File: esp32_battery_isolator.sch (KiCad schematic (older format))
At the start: 78 parts, among them J1 BATT1, J2 Conn_01x04_Female, J3 USB_B_Micro, J4 BATT2, J5 LOAD1, J6 CHGR, J7 LOAD2, J8 LOAD3, J9 Conn_01x03_Male, Q1 MMBT3904, Q10 AONR21321, Q11 AONR21321, Q12 MMBT3904, Q13 AONR21321, Q2 AONR21321, Q3 MMBT3904, Q4 AONR21321, Q5 MMBT3904, Q6 AONR21321, Q7 MMBT3904, Q8 AONR21321, Q9 MMBT3904, SW1 C492887, SW2 C492887, U1 ESP32-WROOM-32D, U3 ADC128D818, U4 CC6903SO-30A, U5 CH330N, U6 CC6903SO-30A, U7 BL9342

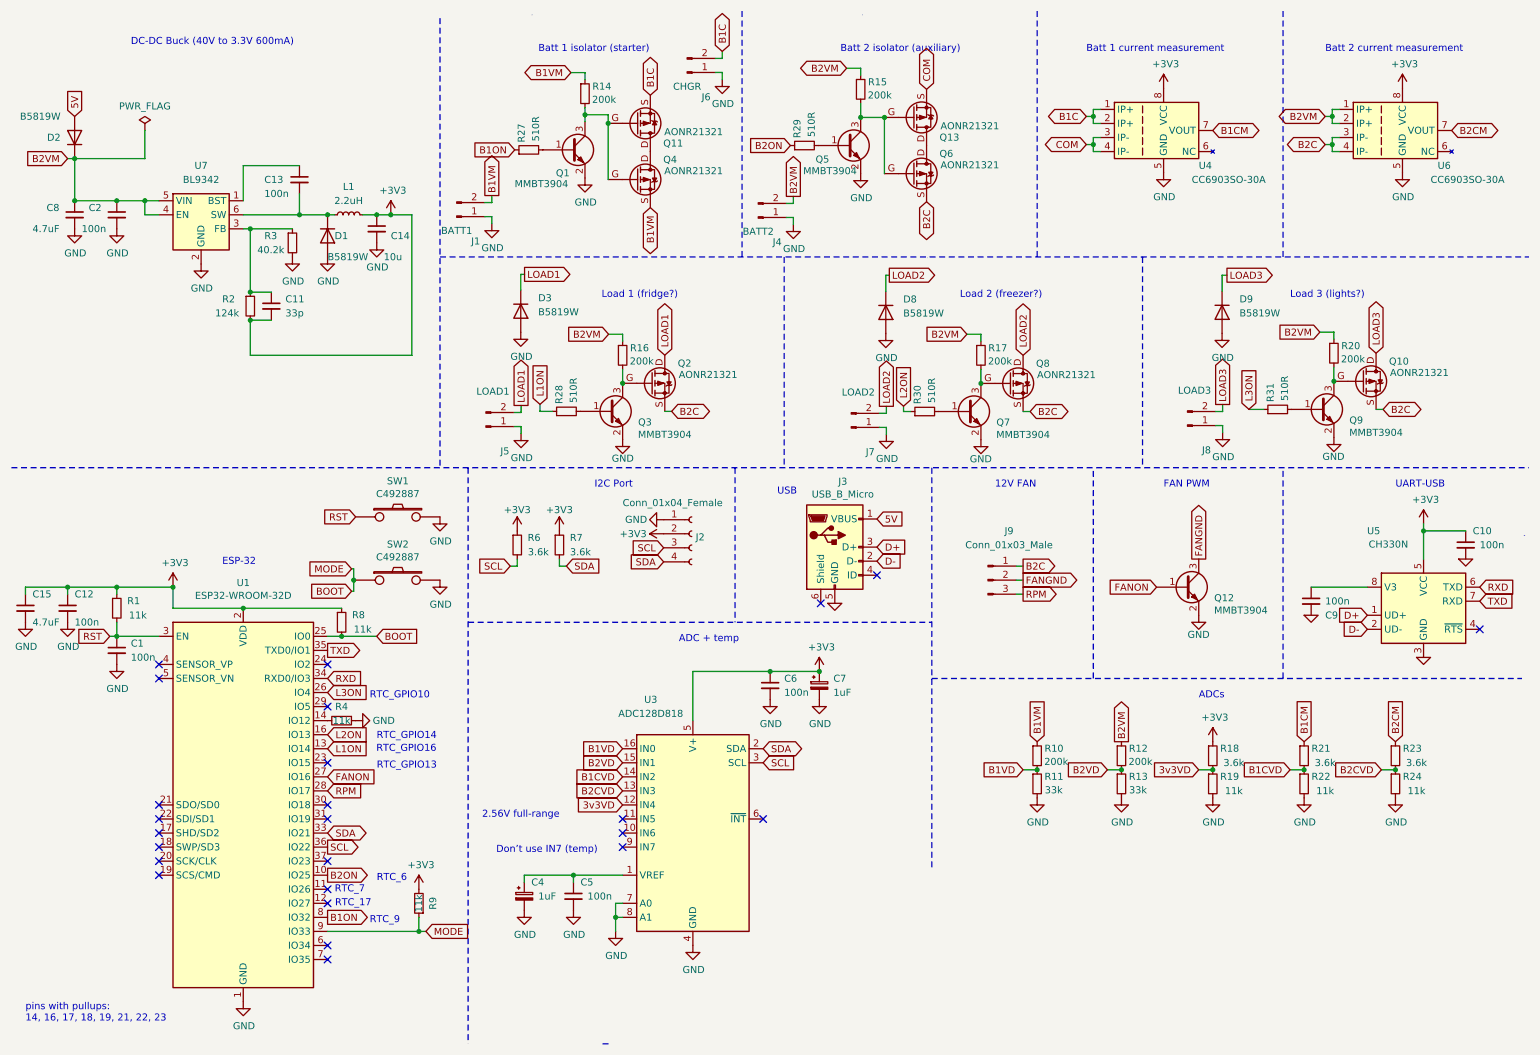
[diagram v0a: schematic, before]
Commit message: REV F - WIP
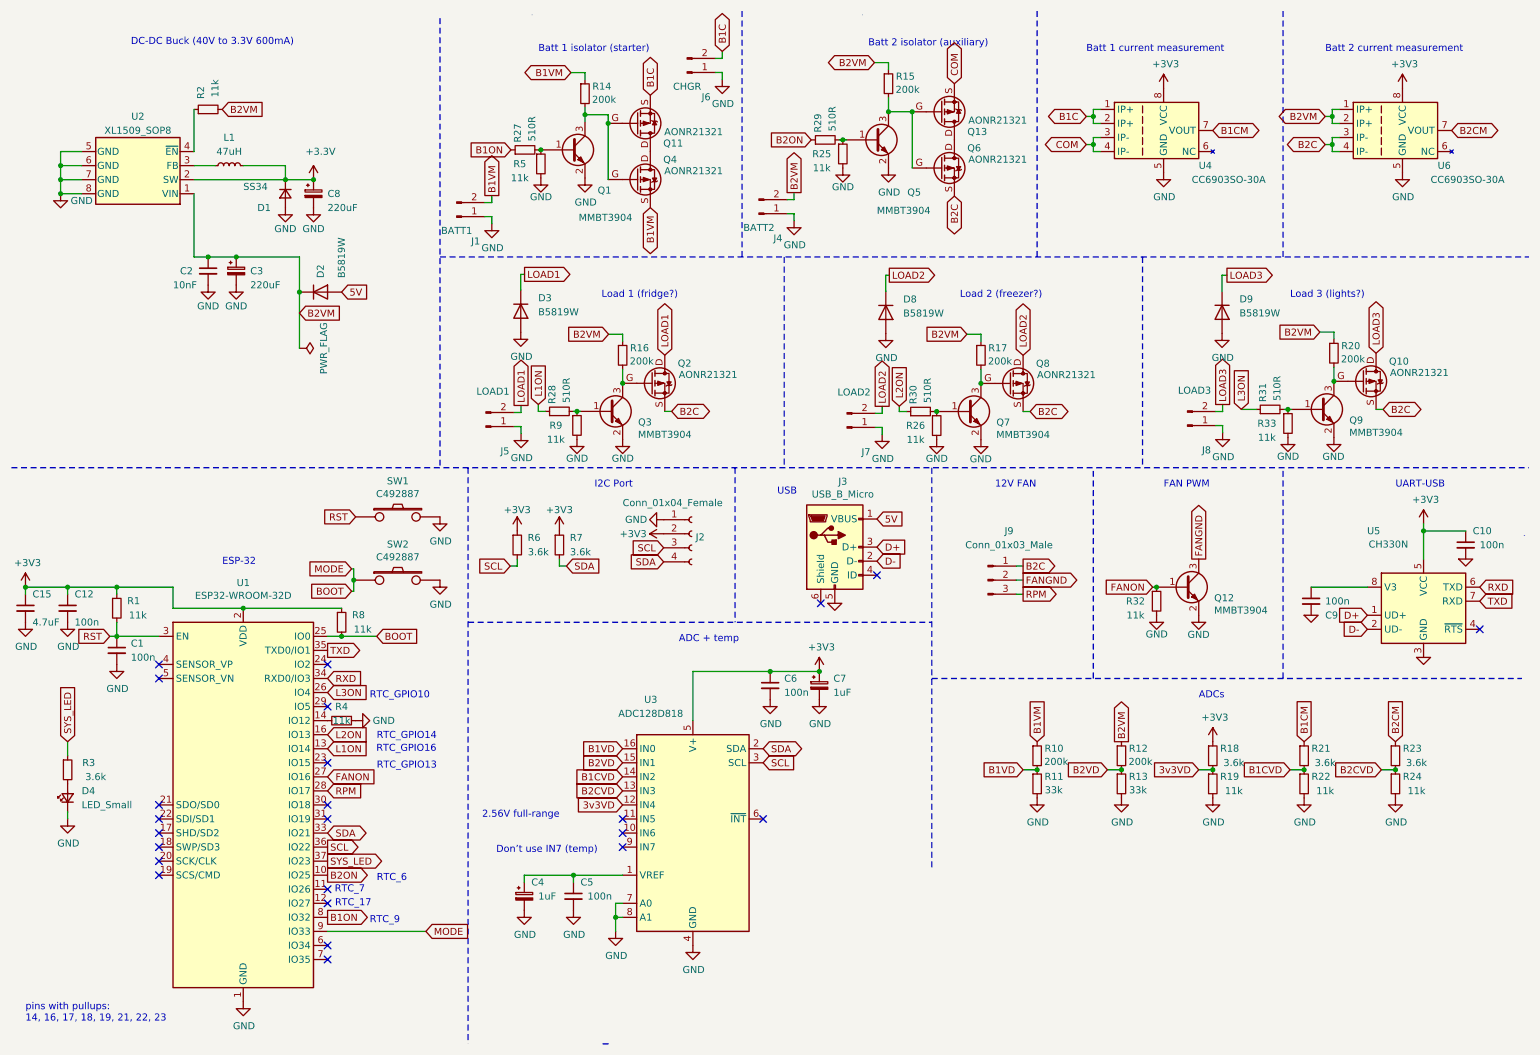
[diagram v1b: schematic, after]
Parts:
- removed C11: 33p, Capacitor_SMD:C_0603_1608Metric, symbol Device:C_Small
- removed C13: 100n, Capacitor_SMD:C_0603_1608Metric, symbol Device:C_Small
- removed C14: 10u, Capacitor_SMD:C_0805_2012Metric, symbol Device:C_Small
- removed C8: 4.7uF, Capacitor_SMD:C_0805_2012Metric, symbol Device:C_Small
- removed D1: B5819W, Diode_SMD:D_SOD-123, symbol Diode:1N4148WS
- removed U7: BL9342, Package_TO_SOT_SMD:SOT-23-6, symbol esp32_battery_isolator-rescue:BL9342-Relay
- added C3: 220uF, Capacitor_SMD:C_Elec_6.3x7.7, symbol Device:CP_Small
- added C8: 220uF, Capacitor_Tantalum_SMD:CP_EIA-3528-15_AVX-H, symbol Device:CP_Small
- added D1: SS34, Diode_SMD:D_SMA, symbol Device:D_Small
- added D4: LED_Small, LED_SMD:LED_0603_1608Metric, symbol Device:LED_Small
- added R25, R26, R32, R33, R5: 11k, Resistor_SMD:R_0603_1608Metric, symbol Device:R_Small
- added U2: XL1509_SOP8, Package_SO:SOIC-8_3.9x4.9mm_P1.27mm, symbol xl1509_sop8:XL1509_SOP8
- C2: value 100n -> 10nF; lcsc_part_number C14663 -> C57112; lcsc_url https://lcsc.com/product-detail/Multilayer-Ceramic-Capacito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 -> (none); package 0603 -> (none)
- L1: value 2.2uH -> 47uH; footprint Inductor_SMD:L_Taiyo-Yuden_NR-30xx -> Inductor_SMD:L_Bourns_SRN6045TA; lcsc_part_number C167747 -> C36414
- R2: value 124k -> 11k; lcsc_part_number C22788 -> C25950; lcsc_url (none) -> https://lcsc.com/product-detail/Chip-Resistor-Surface-Mount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; package (none) -> 0603
- R3: value 40.2k -> 3.6k; lcsc_part_number C12447 -> C22980; lcsc_url (none) -> https://lcsc.com/product-detail/Chip-Resistor-Surface-Mount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; package (none) -> 0603
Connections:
- net +3V3: now also C8.1, D1.1 (K), U2.2 (SW); no longer R2.2, R9.2
- net B2VM: now also R2.2, C3.1, U2.1 (VIN)
- net BOOT: no longer R9.1
- net FANON: now also R32.1
- net GND: now also R9.2, C3.2, C8.2, D1.2 (A), D4.1 (K), R25.2, R26.2, R32.2, R33.2, R5.2, U2.5 (GND), U2.6 (GND), U2.7 (GND), U2.8 (GND); no longer R3.2
- net SYS_LED: now reaches U1.37 (IO23)
- net SYS_LED: now also R3.1
- net at Q1.1 (B), R27.2: now also R5.1
- net at Q5.1 (B), R29.2: now also R25.1
- net at Q3.1 (B), R28.2: now also R9.1
- net at Q7.1 (B), R30.2: now also R26.1
- net at Q9.1 (B), R31.2: now also R33.1
- net at R2.1: now also U2.4 (~EN); no longer R3.1
- net at L1.1: now also U2.3 (FB)
- new net: D4.2 (A), R3.2
- no-connect marks 25 -> 24
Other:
- moved on the sheet: D2, J4, J7, Q13, Q5, Q6, R15, R27, R28, R29, R30, R31
